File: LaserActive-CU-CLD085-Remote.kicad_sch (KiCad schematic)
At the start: 0 parts

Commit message: Initial start
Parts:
- added C1: 100nF, Capacitor_THT:C_Disc_D4.3mm_W1.9mm_P5.00mm, symbol Device:C_Small
- added C2, C3: 10pF, Capacitor_THT:C_Disc_D3.0mm_W1.6mm_P2.50mm, symbol Device:C_Small
- added C4: 47uF, Capacitor_THT:CP_Radial_D5.0mm_P2.00mm, symbol Device:C_Polarized_Small
- added C5: C_Small, Capacitor_THT:C_Disc_D4.3mm_W1.9mm_P5.00mm, symbol Device:C_Small
- added D1: D_Dual_CommonAnode_AKK, Package_TO_SOT_THT:TO-126-3_Vertical, symbol Device:D_Dual_CommonAnode_AKK
- added D3: IRL81A, LED_THT:LED_SideEmitter_Rectangular_W4.5mm_H1.6mm, symbol LED:IRL81A
- added IC1: D6600CS, Package_DIP:DIP-20_W7.62mm_Socket_LongPads, symbol Pioneer:D6600CS
- added K0, K1, K10, K11, K12, K16, K18, K19, K2, K20, K24, K25, K26, K27, K28, K29, K3, K32, K33, K34, K35, K36, K4, K7: Button, Button_Switch_SMD:SW_SPST_CK_KXT3, symbol Switch:SW_Push
- added Q1: NPN, Package_TO_SOT_THT:TO-220-3_Vertical, symbol Simulation_SPICE:NPN
- added R1: 220, Resistor_THT:R_Axial_DIN0204_L3.6mm_D1.6mm_P5.08mm_Horizontal, symbol Device:R_Small
- added X1: Crystal, Crystal:Crystal_HC18-U_Vertical, symbol Device:Crystal
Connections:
- new net: C3.2, IC1.8 (OSC-IN), X1.1
- new net: C2.2, IC1.7 (OSC-OUT), X1.2
- new net: C1.1, IC1.10 (AC)
- new net: D1.2 (K), IC1.3 (S-IN)
- new net: IC1.5 (REM), Q1.2 (B)
- new net: D3.2 (A), Q1.1 (C)
- new net: D3.1 (K), R1.2
- new net COL_1: IC1.14 (K_I0)
- new net COL_2: IC1.13 (K_I1)
- new net COL_3: IC1.12 (K_I2), K16.1, K18.1, K19.1, K20.1
- new net COL_4: IC1.11 (K_I3)
- new net GND: C1.2, C2.1, C3.1, C4.2, C5.2, IC1.9 (VSS), Q1.3 (E)
- new net ROW_1: IC1.2 (K_IO0)
- new net ROW_2: IC1.1 (K_IO1)
- new net ROW_3: IC1.20 (K_IO2)
- new net ROW_4: IC1.19 (K_IO3), K16.2
- new net ROW_5: IC1.18 (K_IO4)
- new net ROW_6: IC1.17 (K_IO5)
- new net ROW_7: IC1.16 (K_IO6)
- new net ROW_8: IC1.15 (K_IO7)
- new net VCC: C4.1, C5.1, IC1.6 (VDD), R1.1
- no-connect marks 0 -> 1

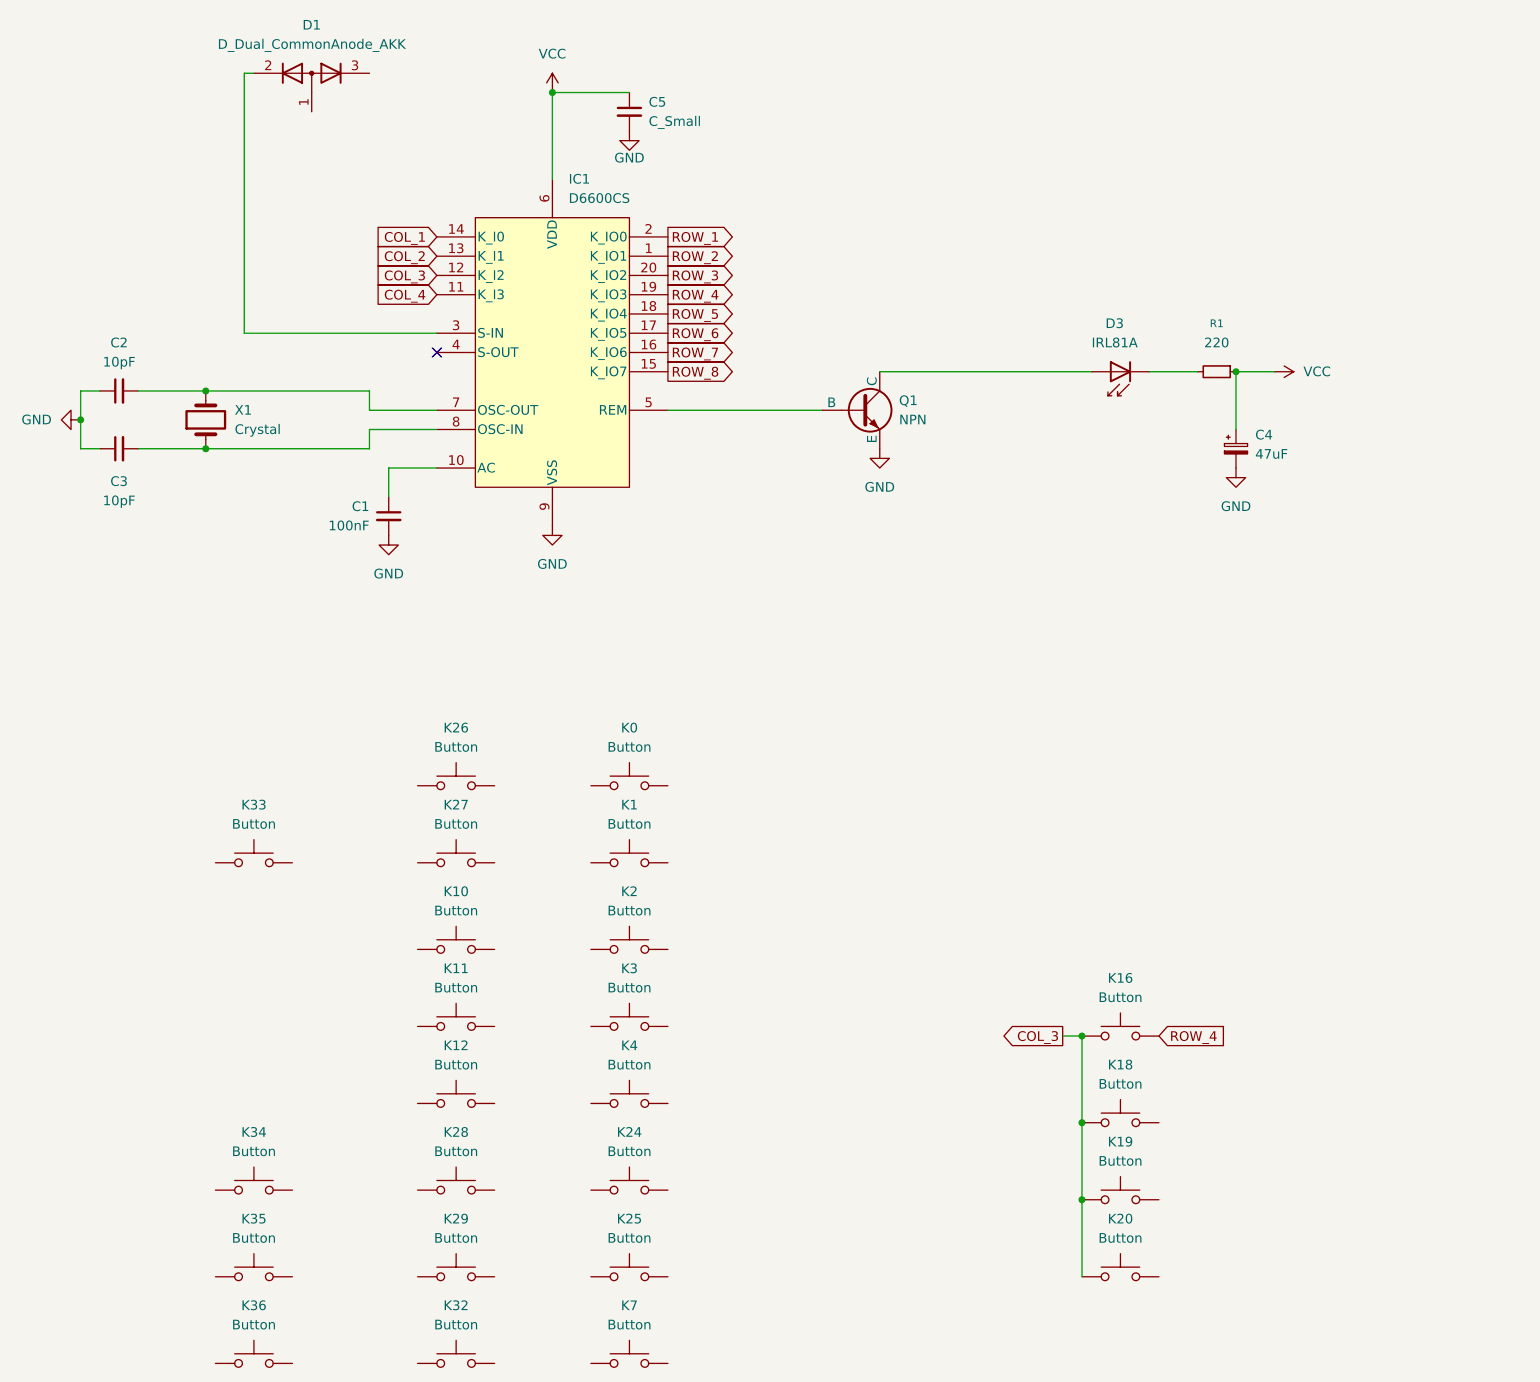
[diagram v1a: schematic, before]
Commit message: Updates
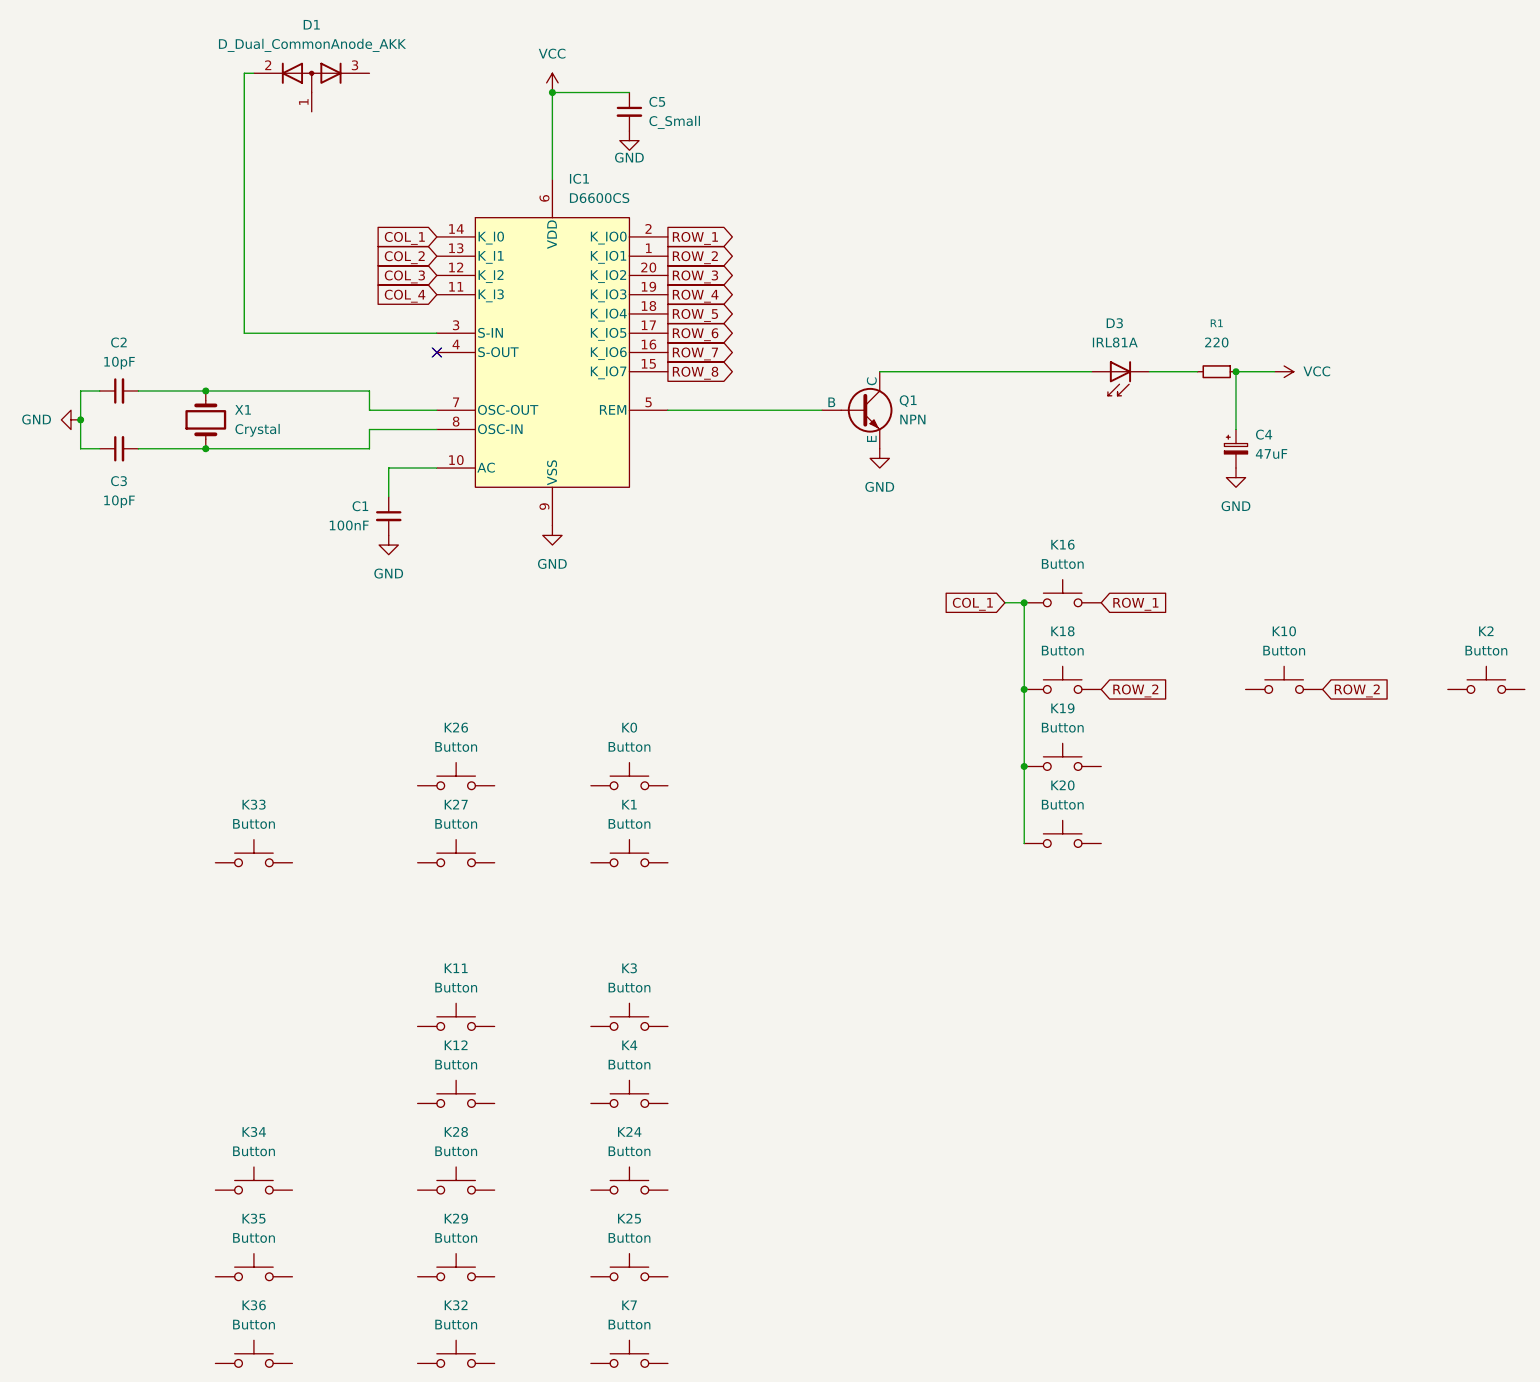
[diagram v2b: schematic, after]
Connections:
- net COL_1: now also K16.1, K18.1, K19.1, K20.1
- net COL_3: no longer K16.1, K18.1, K19.1, K20.1
- net ROW_1: now also K16.2
- net ROW_2: now also K10.2, K18.2
- net ROW_4: no longer K16.2
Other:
- moved on the sheet: K10, K16, K18, K19, K2, K20
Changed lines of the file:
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@@
 	)
 	(junction
-		(at 154.94 171.45)
+		(at 147.32 114.3)
 		(diameter 0)
 		(color 0 0 0 0)
 	)
 	(junction
-		(at 154.94 149.86)
+		(at 147.32 92.71)
 		(diameter 0)
 		(color 0 0 0 0)
 	)
 	(junction
-		(at 154.94 161.29)
+		(at 147.32 104.14)
 		(diameter 0)
 		(color 0 0 0 0)
@@
 	(wire
 		(pts
-			(xy 154.94 161.29) (xy 154.94 171.45)
+			(xy 147.32 104.14) (xy 147.32 114.3)
 		)
 		(stroke
@@
 	(wire
 		(pts
-			(xy 154.94 171.45) (xy 154.94 181.61)
+			(xy 147.32 114.3) (xy 147.32 124.46)
 		)
 		(stroke
@@
 	(wire
 		(pts
-			(xy 152.4 149.86) (xy 154.94 149.86)
+			(xy 144.78 92.71) (xy 147.32 92.71)
 		)
 		(stroke
@@
 	(wire
 		(pts
-			(xy 154.94 149.86) (xy 154.94 161.29)
+			(xy 147.32 92.71) (xy 147.32 104.14)
 		)
 		(stroke
@@
 		)
 	)
-	(global_label "COL_3"
-		(shape output)
-		(at 152.4 149.86 180)
+	(global_label "COL_1"
+		(shape input)
+		(at 144.78 92.71 180)
 		(fields_autoplaced yes)
 		(effects
@@
 		)
 		(property "Intersheetrefs" "${INTERSHEET_REFS}"
-			(at 143.6091 149.86 0)
+			(at 135.9891 92.71 0)
 			(effects
 				(font
@@
 		)
 	)
+	(global_label "ROW_2"
+		(shape input)
+		(at 186.69 104.14 0)
+		(fields_autoplaced yes)
+		(effects
+			(font
+				(size 1.27 1.27)
+			)
+			(justify left)
+		)
+		(property "Intersheetrefs" "${INTERSHEET_REFS}"
+			(at 195.9042 104.14 0)
+			(effects
+				(font
+					(size 1.27 1.27)
+				)
+				(justify left)
+				(hide yes)
+			)
+		)
+	)
 	(global_label "ROW_7"
 		(shape output)
@@
 		)
 	)
-	(global_label "ROW_4"
+	(global_label "ROW_1"
 		(shape input)
-		(at 165.1 149.86 0)
+		(at 157.48 92.71 0)
 		(fields_autoplaced yes)
 		(effects
@@
 		)
 		(property "Intersheetrefs" "${INTERSHEET_REFS}"
-			(at 174.3142 149.86 0)
+			(at 166.6942 92.71 0)
 			(effects
 				(font
@@
 		)
 	)
+	(global_label "ROW_2"
+		(shape input)
+		(at 157.48 104.14 0)
+		(fields_autoplaced yes)
+		(effects
+			(font
+				(size 1.27 1.27)
+			)
+			(justify left)
+		)
+		(property "Intersheetrefs" "${INTERSHEET_REFS}"
+			(at 166.6942 104.14 0)
+			(effects
+				(font
+					(size 1.27 1.27)
+				)
+				(justify left)
+				(hide yes)
+			)
+		)
+	)
 	(global_label "ROW_1"
 		(shape output)
@@
 	(symbol
 		(lib_id "Switch:SW_Push")
-		(at 160.02 149.86 0)
+		(at 152.4 92.71 0)
 		(unit 1)
 		(exclude_from_sim no)
@@
 		(fields_autoplaced yes)
 		(property "Reference" "K16"
-			(at 160.02 142.24 0)
+			(at 152.4 85.09 0)
 			(effects
 				(font
@@
 		)
 		(property "Value" "Button"
-			(at 160.02 144.78 0)
+			(at 152.4 87.63 0)
 			(effects
 				(font
@@
 		)
 		(property "Footprint" "Button_Switch_SMD:SW_SPST_CK_KXT3"
-			(at 160.02 144.78 0)
+			(at 152.4 87.63 0)
 			(effects
 				(font
@@
 		)
 		(property "Datasheet" "~"
-			(at 160.02 144.78 0)
+			(at 152.4 87.63 0)
 			(effects
 				(font
@@
 		)
 		(property "Description" "Push button switch, generic, two pins"
-			(at 160.02 149.86 0)
+			(at 152.4 92.71 0)
 			(effects
 				(font
@@
 	(symbol
 		(lib_id "Switch:SW_Push")
-		(at 160.02 171.45 0)
+		(at 152.4 114.3 0)
 		(unit 1)
 		(exclude_from_sim no)
@@
 		(fields_autoplaced yes)
 		(property "Reference" "K19"
-			(at 160.02 163.83 0)
+			(at 152.4 106.68 0)
 			(effects
 				(font
@@
 		)
 		(property "Value" "Button"
-			(at 160.02 166.37 0)
+			(at 152.4 109.22 0)
 			(effects
 				(font
@@
 		)
 		(property "Footprint" "Button_Switch_SMD:SW_SPST_CK_KXT3"
-			(at 160.02 166.37 0)
+			(at 152.4 109.22 0)
 			(effects
 				(font
@@
 		)
 		(property "Datasheet" "~"
-			(at 160.02 166.37 0)
+			(at 152.4 109.22 0)
 			(effects
 				(font
@@
 		)
 		(property "Description" "Push button switch, generic, two pins"
-			(at 160.02 171.45 0)
+			(at 152.4 114.3 0)
 			(effects
 				(font
@@
 	(symbol
 		(lib_id "Switch:SW_Push")
-		(at 160.02 181.61 0)
+		(at 152.4 124.46 0)
 		(unit 1)
 		(exclude_from_sim no)
@@
 		(fields_autoplaced yes)
 		(property "Reference" "K20"
-			(at 160.02 173.99 0)
+			(at 152.4 116.84 0)
 			(effects
 				(font
@@
 		)
 		(property "Value" "Button"
-			(at 160.02 176.53 0)
+			(at 152.4 119.38 0)
 			(effects
 				(font
@@
 		)
 		(property "Footprint" "Button_Switch_SMD:SW_SPST_CK_KXT3"
-			(at 160.02 176.53 0)
+			(at 152.4 119.38 0)
 			(effects
 				(font
@@
 		)
 		(property "Datasheet" "~"
-			(at 160.02 176.53 0)
+			(at 152.4 119.38 0)
 			(effects
 				(font
@@
 		)
 		(property "Description" "Push button switch, generic, two pins"
-			(at 160.02 181.61 0)
+			(at 152.4 124.46 0)
 			(effects
 				(font
@@
 	(symbol
 		(lib_id "Switch:SW_Push")
-		(at 72.39 138.43 0)
+		(at 181.61 104.14 0)
 		(unit 1)
 		(exclude_from_sim no)
@@
 		(fields_autoplaced yes)
 		(property "Reference" "K10"
-			(at 72.39 130.81 0)
+			(at 181.61 96.52 0)
 			(effects
 				(font
@@
 		)
 		(property "Value" "Button"
-			(at 72.39 133.35 0)
+			(at 181.61 99.06 0)
 			(effects
 				(font
@@
 		)
 		(property "Footprint" "Button_Switch_SMD:SW_SPST_CK_KXT3"
-			(at 72.39 133.35 0)
+			(at 181.61 99.06 0)
 			(effects
 				(font
@@
 		)
 		(property "Datasheet" "~"
-			(at 72.39 133.35 0)
+			(at 181.61 99.06 0)
 			(effects
 				(font
@@
 		)
 		(property "Description" "Push button switch, generic, two pins"
-			(at 72.39 138.43 0)
+			(at 181.61 104.14 0)
 			(effects
 				(font
@@
 	(symbol
 		(lib_id "Switch:SW_Push")
-		(at 160.02 161.29 0)
+		(at 152.4 104.14 0)
 		(unit 1)
 		(exclude_from_sim no)
@@
 		(fields_autoplaced yes)
 		(property "Reference" "K18"
-			(at 160.02 153.67 0)
+			(at 152.4 96.52 0)
 			(effects
 				(font
@@
 		)
 		(property "Value" "Button"
-			(at 160.02 156.21 0)
+			(at 152.4 99.06 0)
 			(effects
 				(font
@@
 		)
 		(property "Footprint" "Button_Switch_SMD:SW_SPST_CK_KXT3"
-			(at 160.02 156.21 0)
+			(at 152.4 99.06 0)
 			(effects
 				(font
@@
 		)
 		(property "Datasheet" "~"
-			(at 160.02 156.21 0)
+			(at 152.4 99.06 0)
 			(effects
 				(font
@@
 		)
 		(property "Description" "Push button switch, generic, two pins"
-			(at 160.02 161.29 0)
+			(at 152.4 104.14 0)
 			(effects
 				(font
@@
 	(symbol
 		(lib_id "Switch:SW_Push")
-		(at 95.25 138.43 0)
+		(at 208.28 104.14 0)
 		(unit 1)
 		(exclude_from_sim no)
@@
 		(fields_autoplaced yes)
 		(property "Reference" "K2"
-			(at 95.25 130.81 0)
+			(at 208.28 96.52 0)
 			(effects
 				(font
@@
 		)
 		(property "Value" "Button"
-			(at 95.25 133.35 0)
+			(at 208.28 99.06 0)
 			(effects
 				(font
@@
 		)
 		(property "Footprint" "Button_Switch_SMD:SW_SPST_CK_KXT3"
-			(at 95.25 133.35 0)
+			(at 208.28 99.06 0)
 			(effects
 				(font
@@
 		)
 		(property "Datasheet" "~"
-			(at 95.25 133.35 0)
+			(at 208.28 99.06 0)
 			(effects
 				(font
@@
 		)
 		(property "Description" "Push button switch, generic, two pins"
-			(at 95.25 138.43 0)
+			(at 208.28 104.14 0)
 			(effects
 				(font
